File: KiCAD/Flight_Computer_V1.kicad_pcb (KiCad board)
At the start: 4 copper layers, 36.8 x 63.5 mm, 52 parts, among them IC1 ESP32-S2-MINI-2-N4R2, J1 Conn_01x04_Pin, J2 Conn_01x04_Pin, J3 Conn_01x06_Pin, J4 Conn_02x04_Odd_Even, Q1 PMOS, Q2 NMOS, Q3 NMOS, SW1 PTS636 SM50J SMTR LFS, U1 W25Q16JVSSIQ, U2 MAX-M10M-00B, U4 BMI088, U5 MMC5983MA, U6 MS560702BA03-50

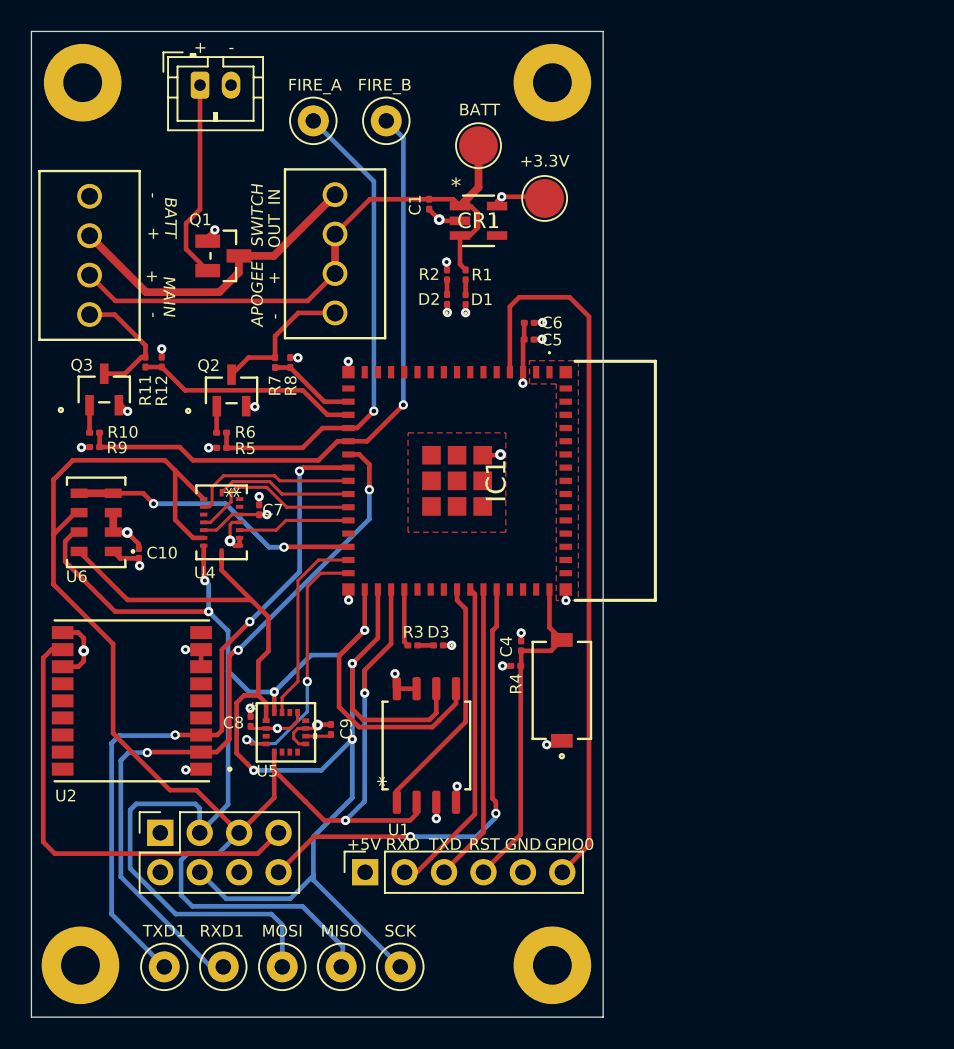
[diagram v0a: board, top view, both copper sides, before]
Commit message: Changes
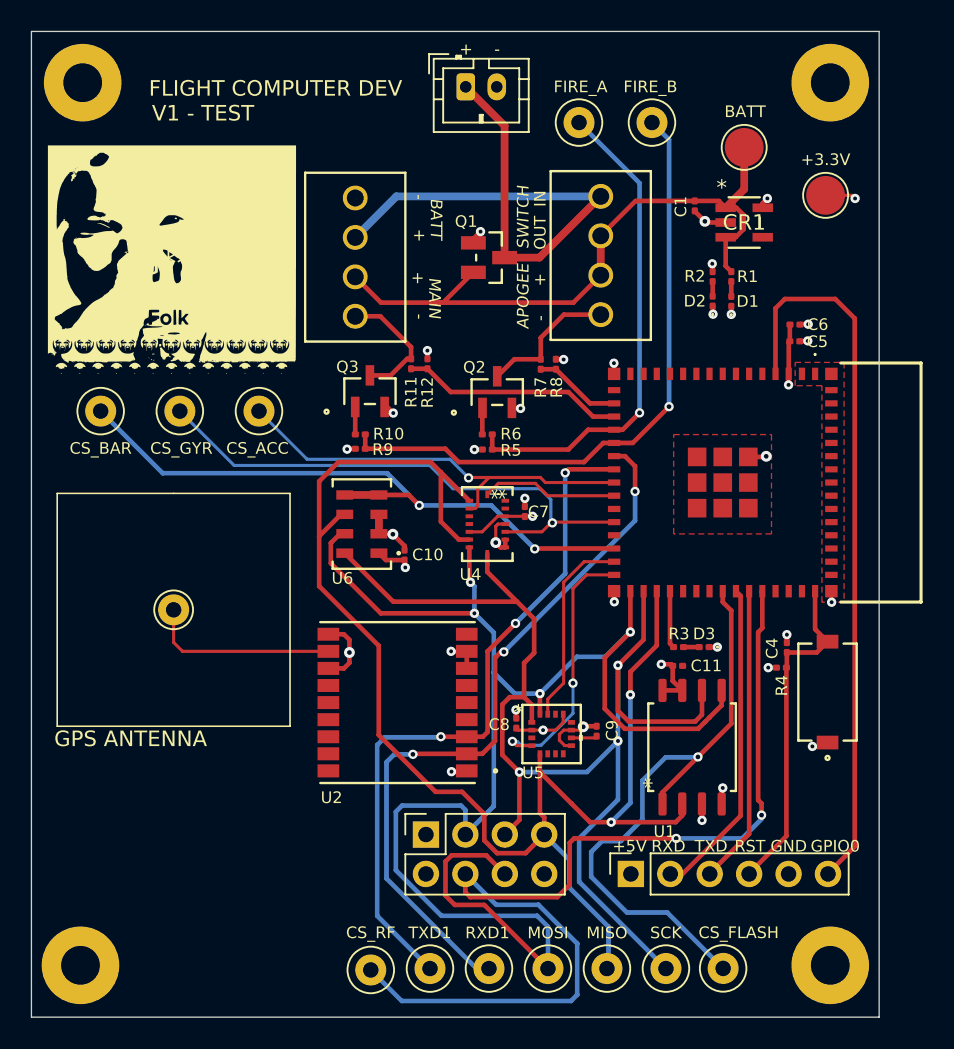
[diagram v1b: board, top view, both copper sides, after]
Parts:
- added C11: 0.1uF, Capacitor_SMD:C_0201_0603Metric, F.Cu at (56.9, 56.1)
- added G***: LOGO, graphics:theone, F.Cu at (24.3, 30.2)
- added GPS_ANT: Pin_D1.0mm_L10.0mm, Connector_Pin:Pin_D1.0mm_L10.0mm, F.Cu at (24.4, 52.5)
- added TP10: TestPoint, TestPoint:TestPoint_Loop_D1.80mm_Drill1.0mm_Beaded, F.Cu at (29.9, 39.7)
- added TP11: TestPoint, TestPoint:TestPoint_Loop_D1.80mm_Drill1.0mm_Beaded, F.Cu at (24.8, 39.7)
- added TP12: TestPoint, TestPoint:TestPoint_Loop_D1.80mm_Drill1.0mm_Beaded, F.Cu at (19.7, 39.7)
- added TP14: TestPoint, TestPoint:TestPoint_Loop_D1.80mm_Drill1.0mm_Beaded, F.Cu at (59.8, 75.6)
- added TP15: TestPoint, TestPoint:TestPoint_Loop_D1.80mm_Drill1.0mm_Beaded, F.Cu at (37.1, 75.7)
- moved TP1 18.1 mm to (66.4, 25.8)
- moved H3 17.9 mm to (66.7, 18.5)
- moved H4 17.9 mm to (66.7, 75.4)
- moved SW1 17.1 mm to (66.5, 57.8)
- moved BT1 17.1 mm to (43.2, 18.8)
- moved C1 17.1 mm to (58.0, 26.5)
- moved C4 17.1 mm to (63.9, 54.9)
- moved C5 17.1 mm to (64.4, 35.2)
- moved C7 17.1 mm to (47.0, 46.2)
- moved C8 17.1 mm to (46.5, 59.8)
- moved C9 17.1 mm to (51.7, 60.3)
- moved D1 17.1 mm to (60.3, 32.6)
- moved D2 17.1 mm to (59.1, 32.6)
- moved D3 17.1 mm to (58.6, 54.9)
- moved IC1 17.1 mm to (59.8, 44.3)
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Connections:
- BT1 pad 1: LiPO -> RAW_BATT
- IC1 pad 25: GYRO_INT -> unconnected-(IC1-IO21-Pad25)
- IC1 pad 41: CS_GPS -> CS_RF
- IC1 pad 42: unconnected-(IC1-GND_4-Pad42) -> GND
- IC1 pad 43: unconnected-(IC1-GND_5-Pad43) -> GND
- J1 pad 1: MOS_LIPO -> RAW_BATT
- J2 pad 2: MOS_LIPO -> RAW_BATT
- J4 pad 3: MOSI -> GD00
- J4 pad 4: SCK -> CS_RF
- J4 pad 5: MISO -> SCK
- J4 pad 6: unconnected-(J4-Pin_6-Pad6) -> MOSI
- J4 pad 7: GD0 -> MISO
- J4 pad 8: CS_GPS -> unconnected-(J4-Pin_8-Pad8)
- Q1 pad 2: LiPO -> +BATT
- Q1 pad 3: MOS_LIPO -> RAW_BATT
- U2 pad 11: GD0 -> Net-(GPS_ANT1-Pin_1)
- U4 pad 12: GYRO_INT -> unconnected-(U4-INT3-Pad12)
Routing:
- net CS_RF: track 0.00 -> 65.7 mm, vias 0 -> 2
- net RAW_BATT: track 0.00 -> 37.3 mm
- net CS_GPS: track 30.4 -> 0.00 mm, vias 2 -> 0
- net GD0: track 29.4 -> 0.00 mm
- net CS_GYRO: track 7.27 -> 35.1 mm, vias 0 -> 1
- net CS_FLASH: track 15.8 -> 39.1 mm, vias 0 -> 1
- net CS_BARO: track 18.8 -> 41.8 mm
- net MOS_LIPO: track 21.0 -> 0.00 mm
- net CS_ACCEL: track 10.9 -> 27.5 mm, vias 0 -> 1
- net MOSI: track 87.3 -> 102.5 mm
- net LiPO: track 12.9 -> 0.00 mm
- net Net-(U2-RF_IN): track 0.00 -> 12.3 mm
- net GYRO_INT: track 11.1 -> 0.00 mm
- net MISO: track 102.7 -> 97.0 mm
- net SCK: track 85.9 -> 81.7 mm
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- added copper zone on In2.Cu, net +3.3V
- added copper zone on In1.Cu, net GND
- removed copper zone on In1.Cu, net +3.3V
- removed copper zone on In2.Cu, net GND
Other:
- board size 36.8 x 63.5 mm -> 54.6 x 63.5 mm
- board text added: "CS_ACC"
- board text added: "CS_BAR"
- board text added: "CS_FLASH"
- board text added: "CS_GYR"
- board text added: "CS_RF"
- board text added: "FLIGHT COMPUTER DEV"
- board text added: "GPS ANTENNA"
- board text added: "V1 - TEST"
